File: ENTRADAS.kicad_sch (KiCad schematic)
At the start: 37 parts, among them IC6 ILD206T, J13 1728810000, J8 1728840000, J9 1728840000, U23 ILD206T, U26 ILD206T, U27 ILD206T, U42 MAX3227

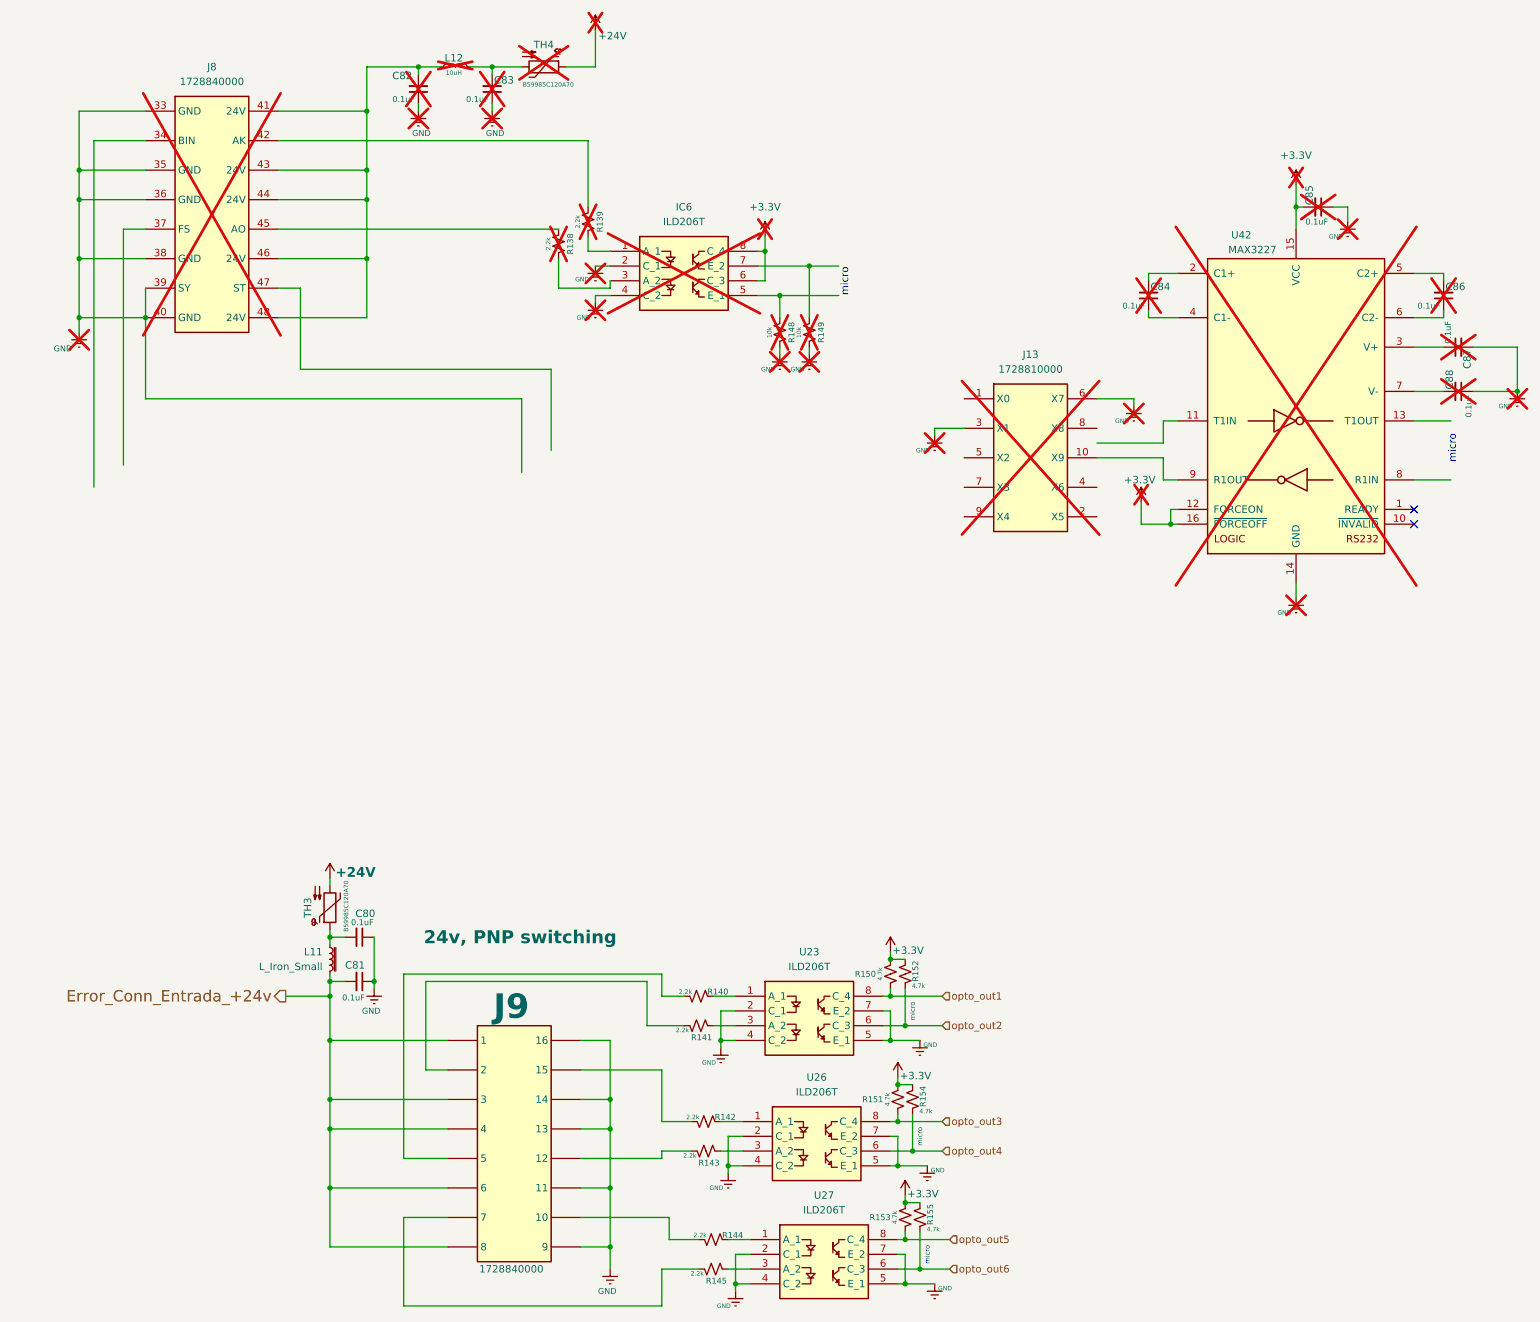
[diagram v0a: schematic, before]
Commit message: 26-05-26
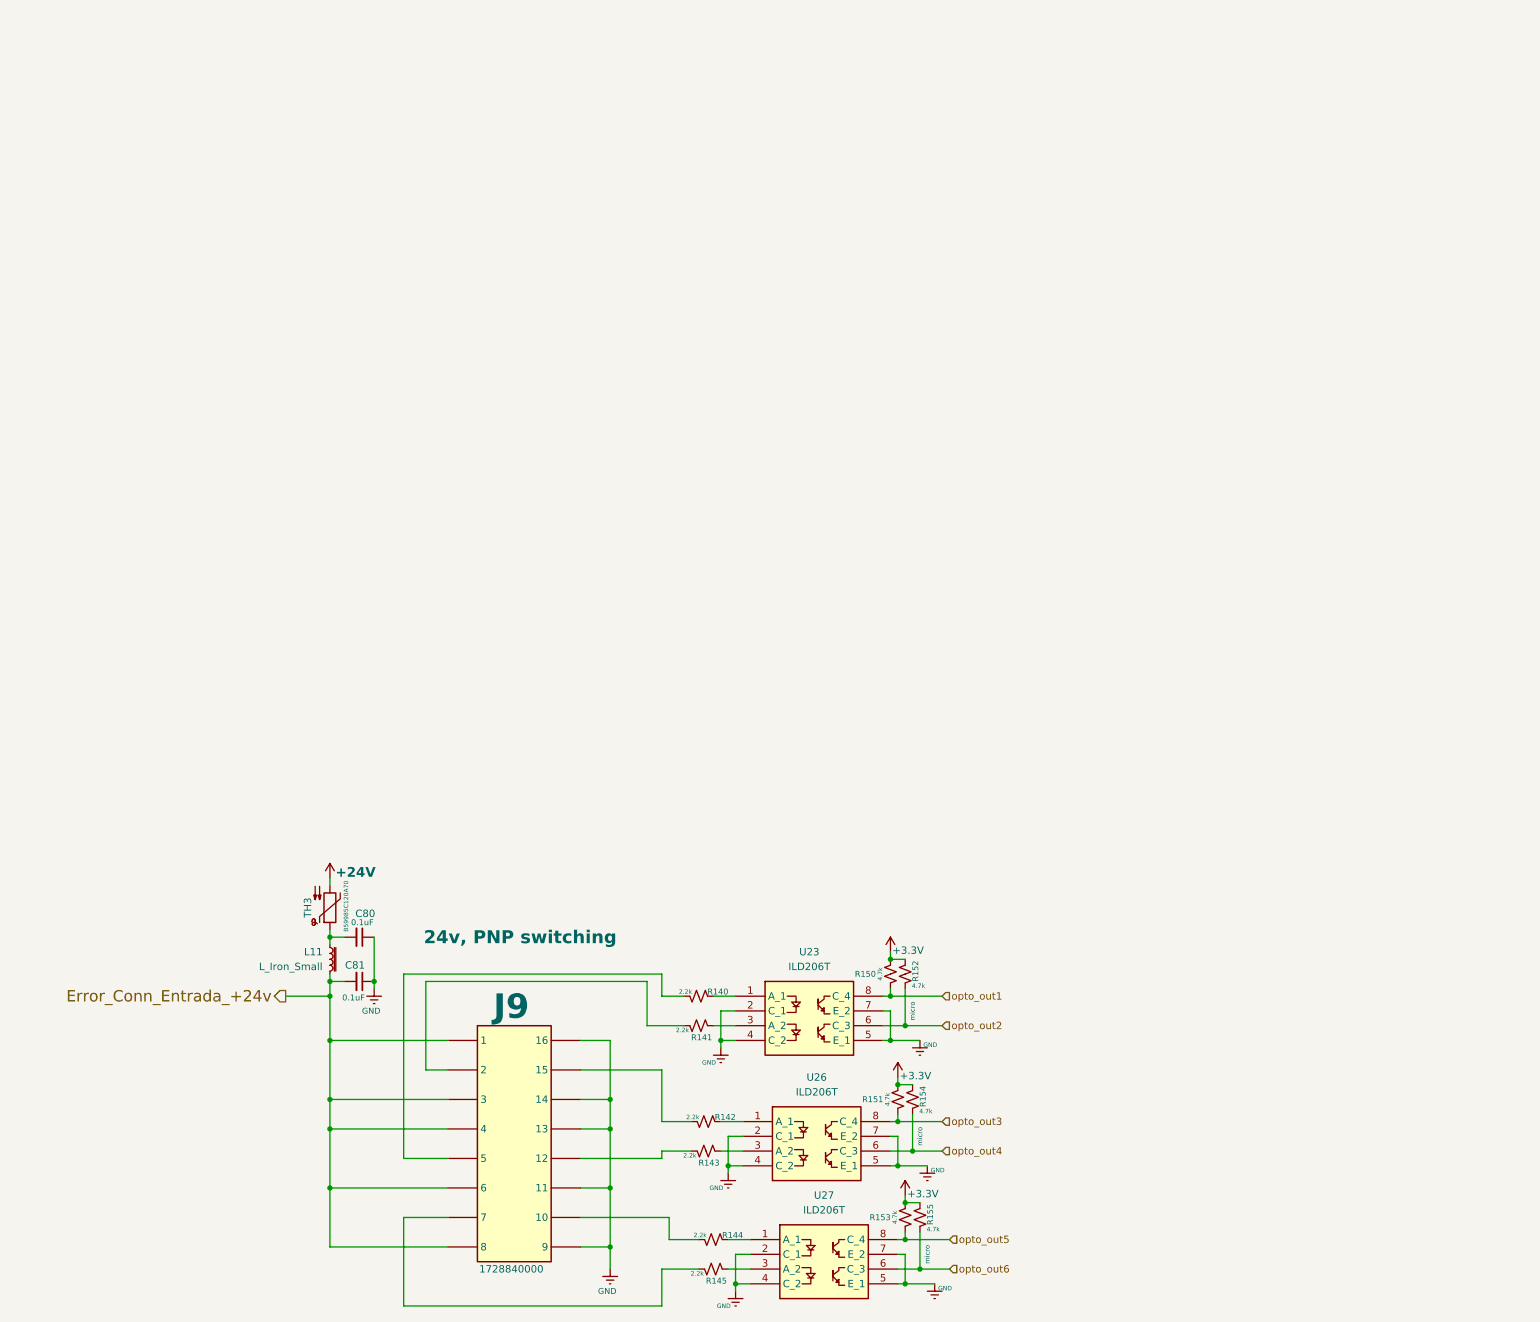
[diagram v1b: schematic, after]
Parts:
- removed C82, C83, C84, C85, C86, C87, C88: 0.1uF, Capacitor_SMD:C_0603_1608Metric_Pad1.08x0.95mm_HandSolder, symbol Device:C_Small
- removed IC6: ILD206T, SOIC:SOIC 8, symbol OPTOACOPLADORES:ILD206T
- removed J13: 1728810000, CONECTORES GRACIDA:1728810000, symbol CONECTORES GRACIDA:1728810000
- removed J8: 1728840000, CONECTORES GRACIDA:16POS-2LINEAS-3.5PITCH, symbol CONECTORES GRACIDA:1728840000_33-48
- removed L12: 10uH, Inductor_SMD:L_0603_1608Metric_Pad1.05x0.95mm_HandSolder, symbol Device:L_Small
- removed R138, R139: 2.2k, Capacitor_SMD:C_0603_1608Metric_Pad1.08x0.95mm_HandSolder, symbol Device:R_Small_US
- removed R148, R149: 10k, Capacitor_SMD:C_0603_1608Metric_Pad1.08x0.95mm_HandSolder, symbol Device:R_Small_US
- removed TH4: B59985C120A70, TERMISTORES GRACIDA:B59985C0120A070, symbol Device:Thermistor_PTC
- removed U42: MAX3227, Package_SO:SSOP-16_5.3x6.2mm_P0.65mm, symbol Interface_UART:MAX3227
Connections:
- no-connect marks 2 -> 0
